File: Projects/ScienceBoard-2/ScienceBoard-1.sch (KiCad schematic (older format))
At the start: 79 parts, among them J1 Conn_01x08, J10 Conn_01x04, J11 Conn_01x02, J2 Laser 1, J3 Conn_01x04, J4 Conn_01x02, J5 Conn_01x02, J6 76825-0006, J7 Conn_01x02, J8 Conn_01x06, J9 Conn_01x02, K1 J115F11AH12VDCS61.5U, Q1 BTN8982TA, Q2 BTN8982TA, Q3 SUD50P04-08, Q4 TIP35CW, Q5 FMMT634Q, Q6 SST4401, Q7 Q_PNP_BCE, Q8 NSS60201LT1G, U1 DRV8834, U3 NCP57302, U9 DRV8834

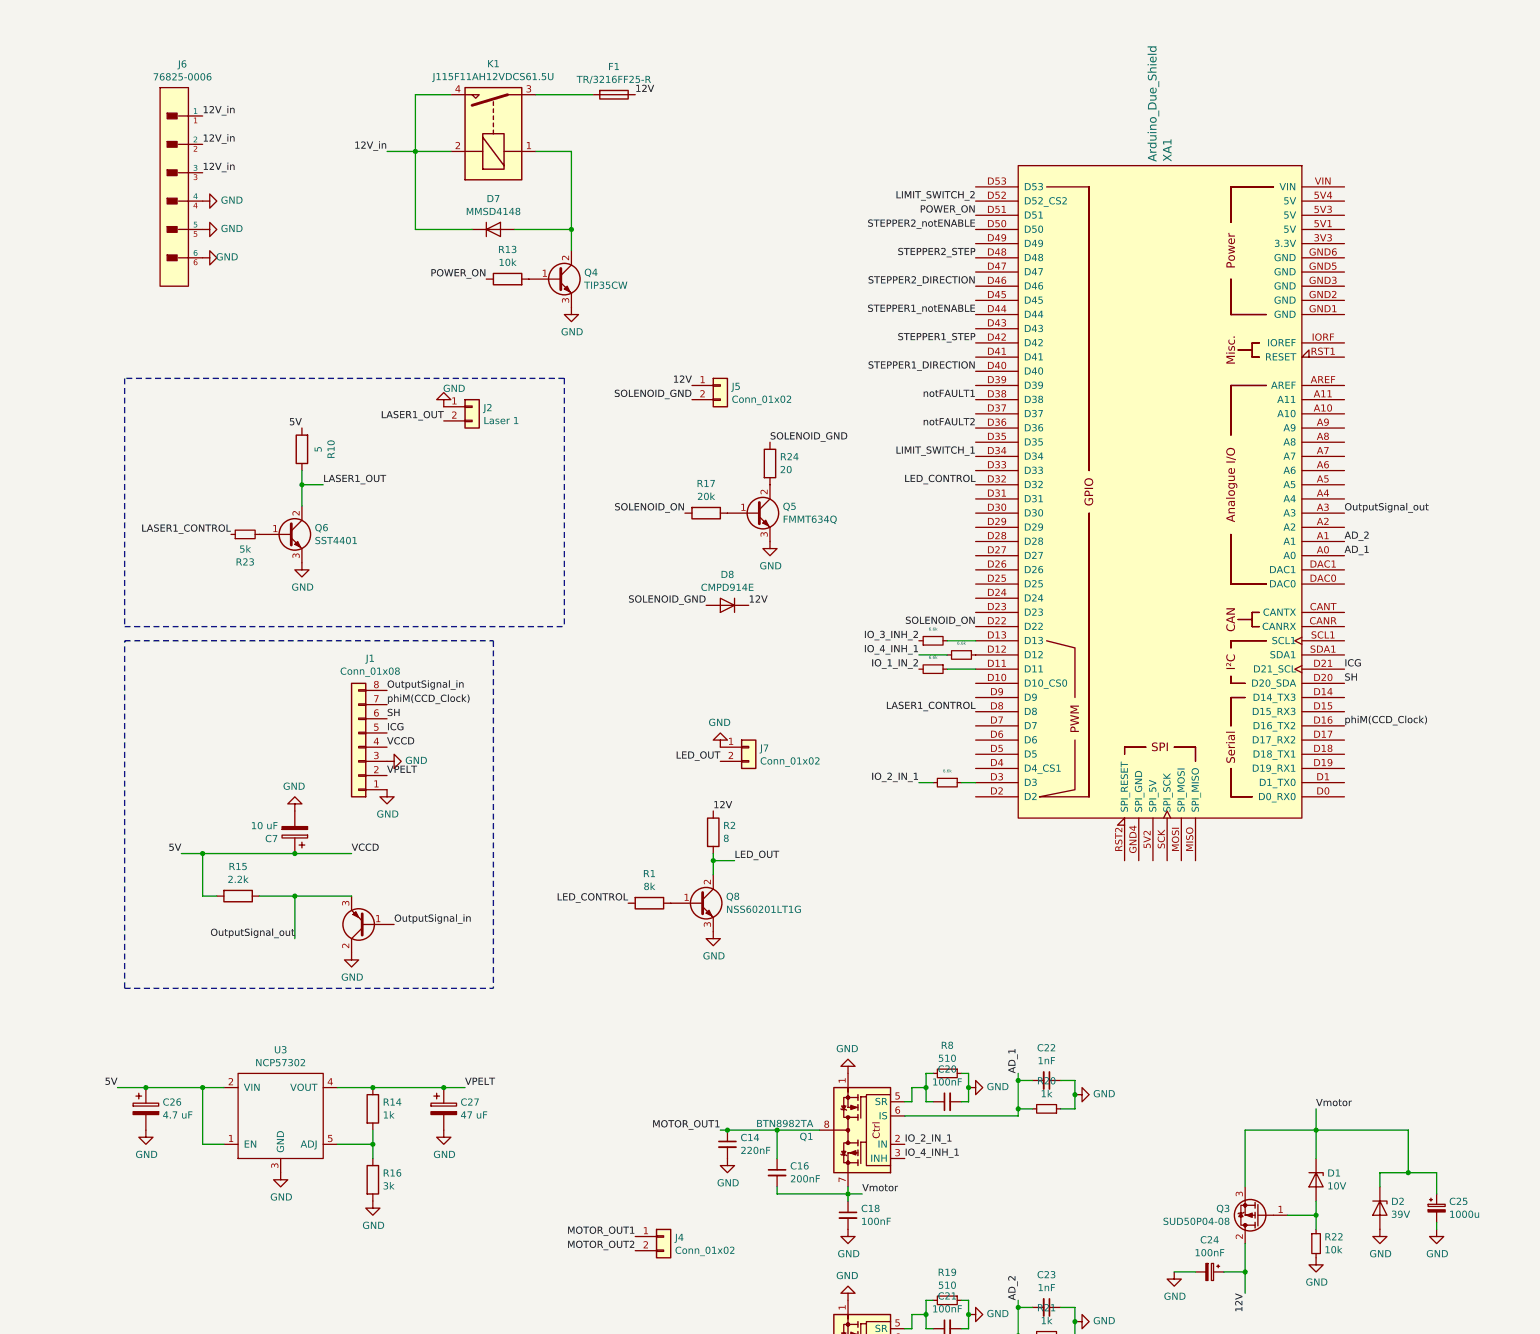
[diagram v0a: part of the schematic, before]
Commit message: Add files via upload
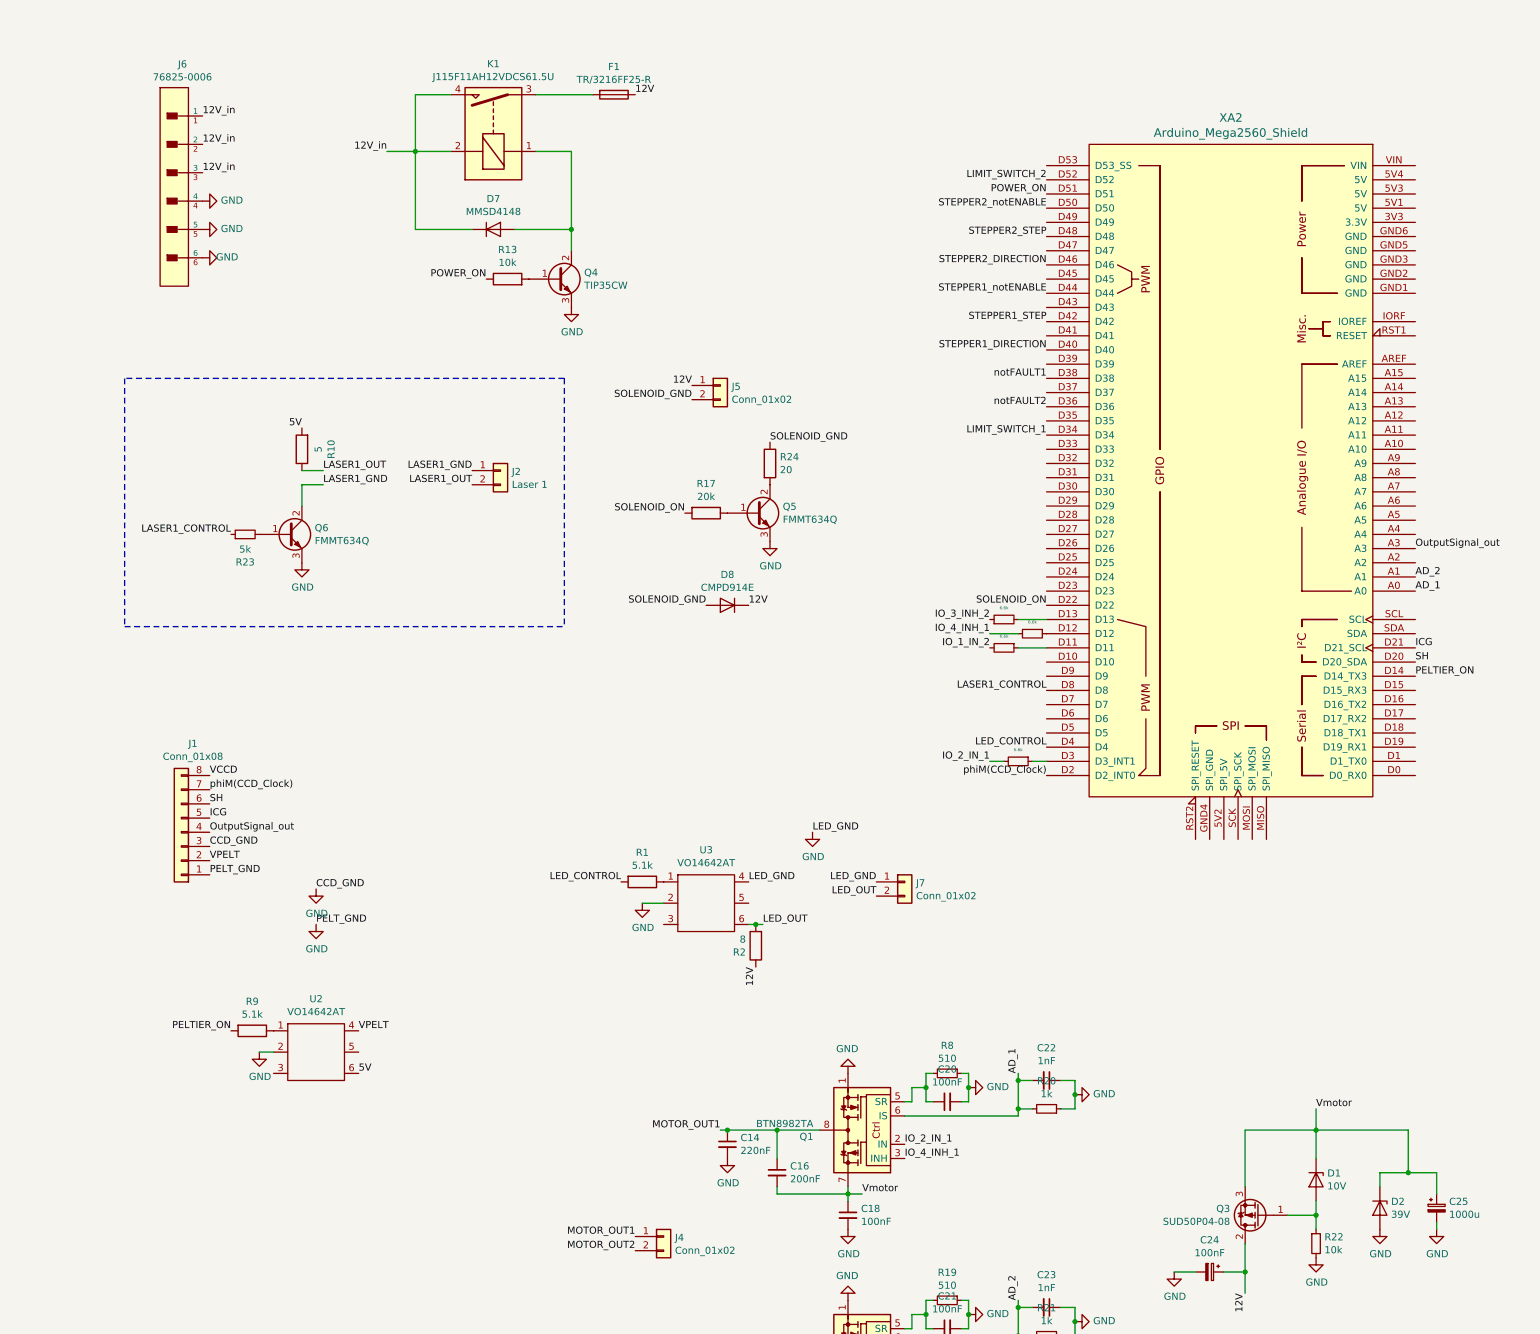
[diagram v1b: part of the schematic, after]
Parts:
- removed C26: 4.7 uF, Capacitor_SMD:C_0402_1005Metric, symbol Device:CP
- removed C27: 47 uF, Capacitor_SMD:C_0402_1005Metric, symbol Device:CP
- removed C7: 10 uF, Capacitor_SMD:CP_Elec_3x5.3, symbol Device:CP
- removed Q7: Q_PNP_BCE, Package_TO_SOT_SMD:SOT-23, symbol Device:Q_PNP_BCE
- removed Q8: NSS60201LT1G, Package_TO_SOT_SMD:SOT-23, symbol Device:Q_NPN_BCE
- removed R14: 1k, Resistor_SMD:R_0402_1005Metric, symbol Device:R
- removed R15: 2.2k, Resistor_SMD:R_0402_1005Metric, symbol Device:R
- removed R16: 3k, Resistor_SMD:R_0402_1005Metric, symbol Device:R
- removed U3: NCP57302, Package_TO_SOT_SMD:TO-252-5_TabPin3, symbol Regulator_Linear:NCP57302
- removed XA1: Arduino_Due_Shield, Arduino:Arduino_Due_Shield, symbol arduino:Arduino_Due_Shield
- added R9: 5.1k, Resistor_SMD:R_0402_1005Metric, symbol Device:R
- added U2, U3: VO14642AT, Package_DIP:VO14642AT, symbol Relay_SolidState:VO14642AT
- added XA2: Arduino_Mega2560_Shield, Arduino:Arduino_Mega2560_Shield, symbol arduino:Arduino_Mega2560_Shield
- Q6: value SST4401 -> FMMT634Q
- R1: value 8k -> 5.1k
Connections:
- net 5V: now also U2.6; no longer J1.4 (Pin_4)
- net AD_1: now also XA2.A0
- net AD_2: now also XA2.A1
- net GND: now also U2.2, U3.2, U3.4; no longer J2.1 (Pin_1)
- net ICG: now also XA2.D21 (D21_SCL)
- net LASER1_CONTROL: now also XA2.D8
- net LASER1_OUT: no longer Q6.2 (C)
- net LED_CONTROL: now also XA2.D4
- net LED_OUT: now also U3.6
- net LIMIT_SWITCH_1: now also XA2.D34
- net LIMIT_SWITCH_2: now also XA2.D52
- net OutputSignal_out: now also J1.4 (Pin_4), XA2.A3
- net POWER_ON: now also XA2.D51
- net SH: now also XA2.D20 (D20_SDA)
- net SOLENOID_ON: now also XA2.D22
- net STEPPER1_DIRECTION: now also XA2.D40
- net STEPPER1_STEP: now also XA2.D42
- net STEPPER1_notENABLE: now also XA2.D44
- net STEPPER2_DIRECTION: now also XA2.D46
- net STEPPER2_STEP: now also XA2.D48
- net STEPPER2_notENABLE: now also XA2.D50
- net VPELT: now also U2.4
- net notFAULT1: now also XA2.D38
- net notFAULT2: now also XA2.D36
- net phiM(CCD_Clock): now also XA2.D2 (D2_INT0)
- net at R32.1: now also XA2.D11
- net at R34.1: now also XA2.D12
- net at R31.2: now also XA2.D13
- net at R33.1: now also XA2.D3 (D3_INT1)
- net at R1.1: now also U3.1
- net OutputSignal_in renamed VCCD
- new net: R9.1, U2.1
- new net LASER1_GND: J2.1 (Pin_1), Q6.2 (C)
- new net PELTIER_ON: R9.2, XA2.D14 (D14_TX3)
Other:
- moved on the sheet: J1, J2, J7, R1, R2
